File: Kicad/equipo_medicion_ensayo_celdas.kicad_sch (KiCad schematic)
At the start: 0 parts

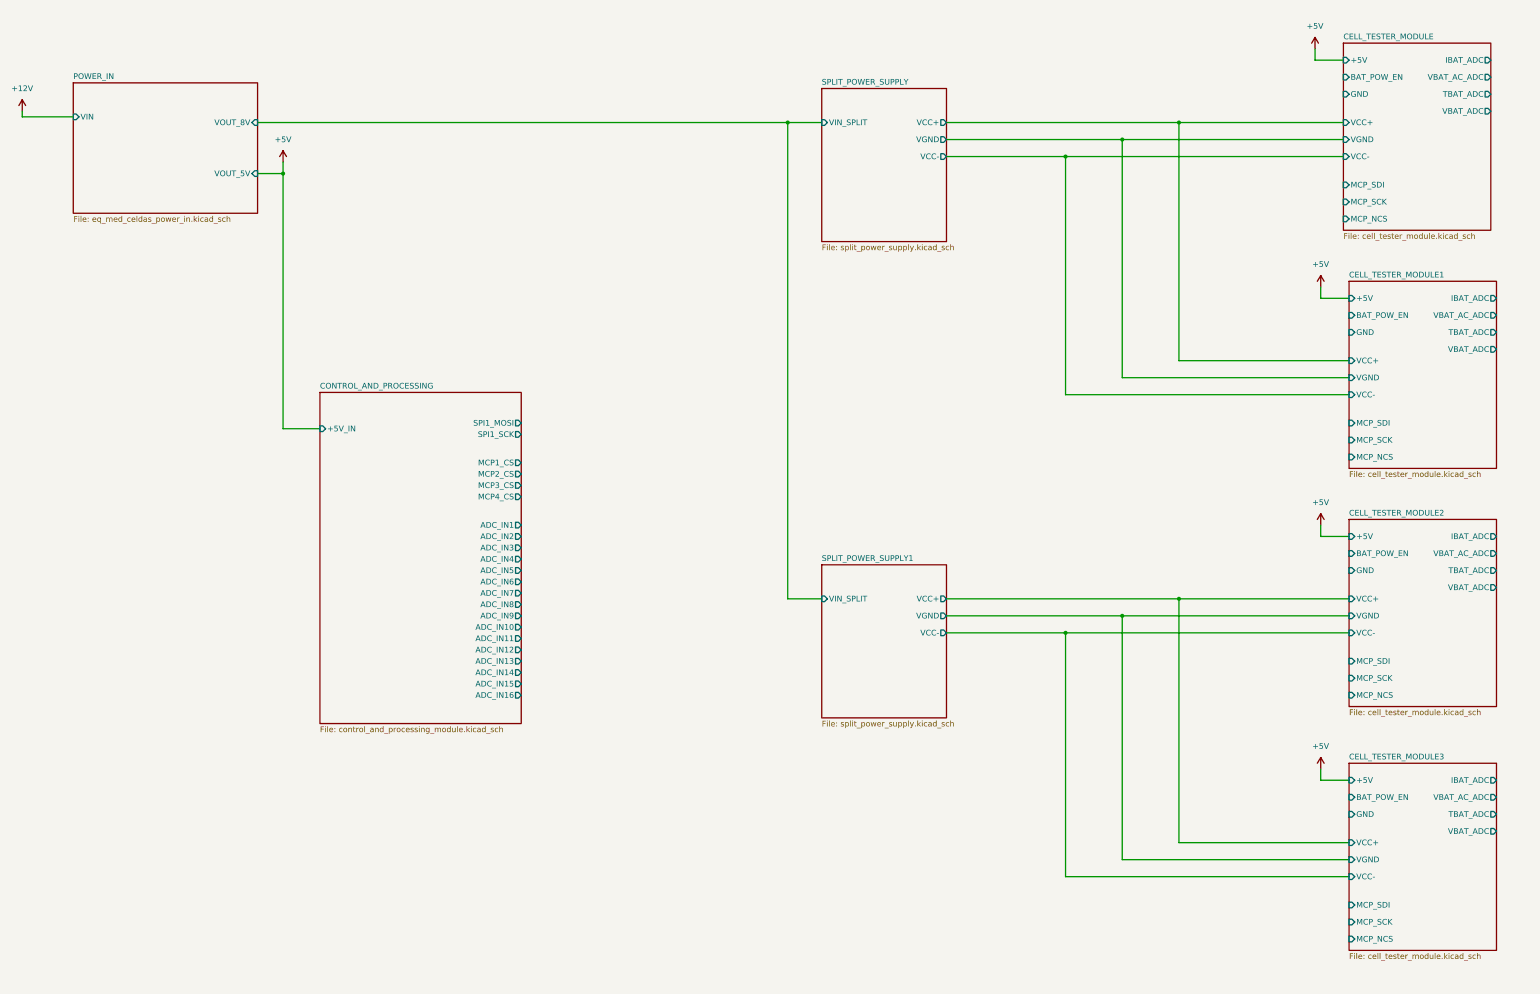
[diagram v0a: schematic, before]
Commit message: Avances en el esquemático de Kicad.
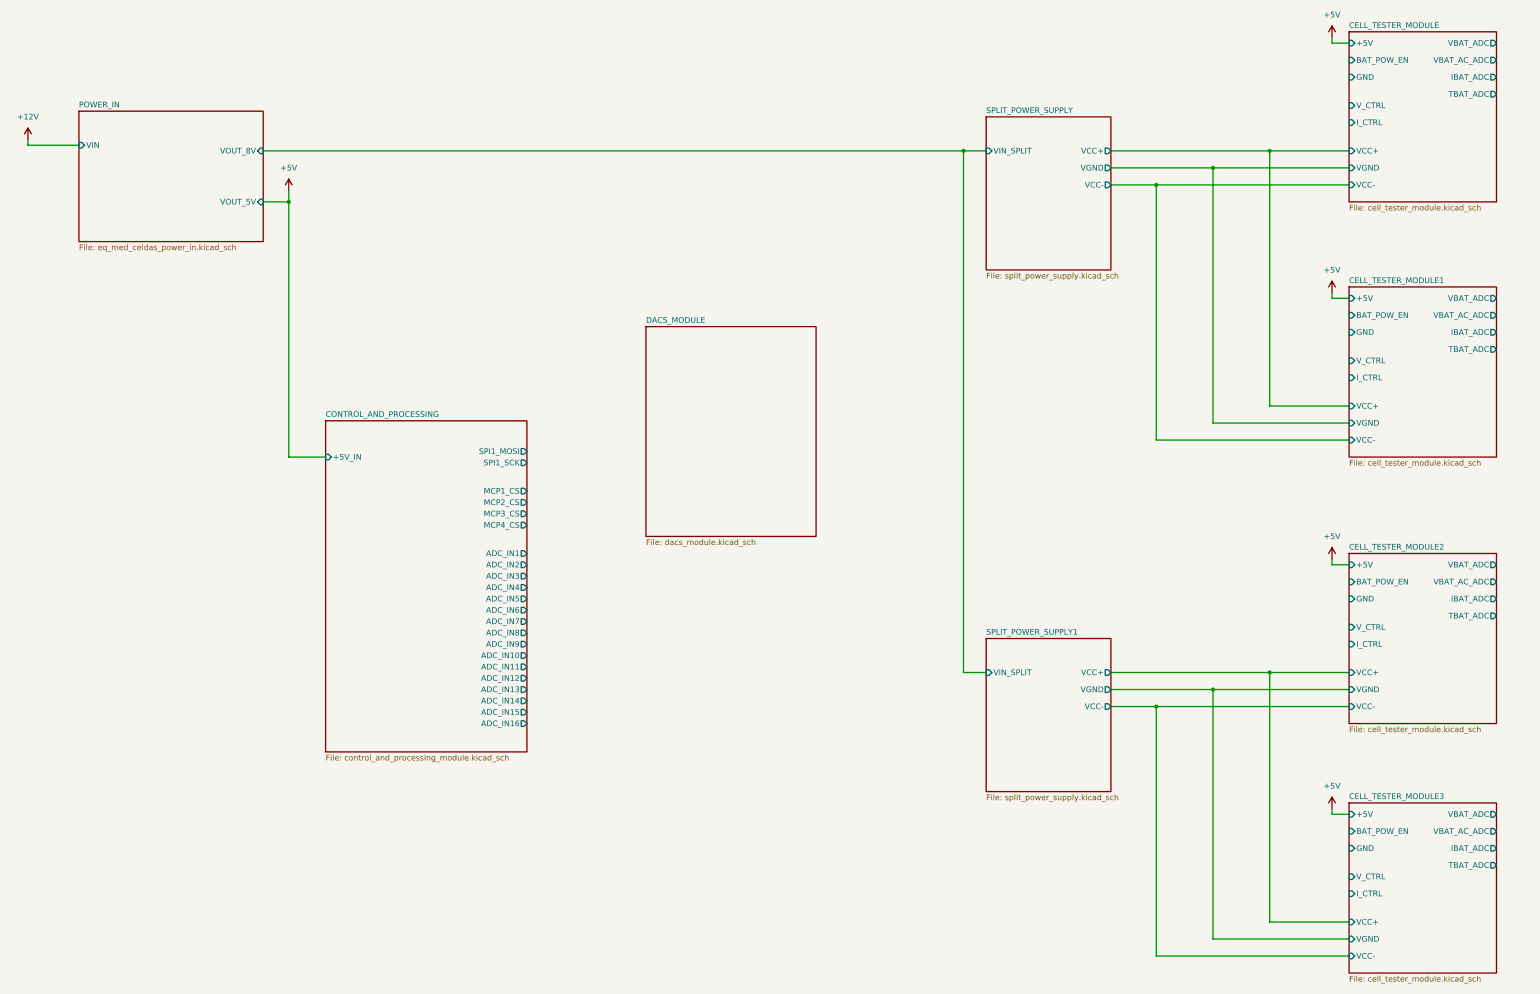
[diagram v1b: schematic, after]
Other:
- added sheet DACS_MODULE (dacs_module.kicad_sch)
- sheet CELL_TESTER_MODULE ports: added I_CTRL, V_CTRL; removed MCP_NCS, MCP_SCK, MCP_SDI
- sheet CELL_TESTER_MODULE1 ports: added I_CTRL, V_CTRL; removed MCP_NCS, MCP_SCK, MCP_SDI
- sheet CELL_TESTER_MODULE2 ports: added I_CTRL, V_CTRL; removed MCP_NCS, MCP_SCK, MCP_SDI
- sheet CELL_TESTER_MODULE3 ports: added I_CTRL, V_CTRL; removed MCP_NCS, MCP_SCK, MCP_SDI
